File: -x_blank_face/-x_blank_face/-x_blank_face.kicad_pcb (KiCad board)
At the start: 2 copper layers, 87 x 326.5 mm, 29 parts, among them J1 Conn_01x08_Pin, J2 Conn_01x02_Pin, J3 Conn_01x02_Pin

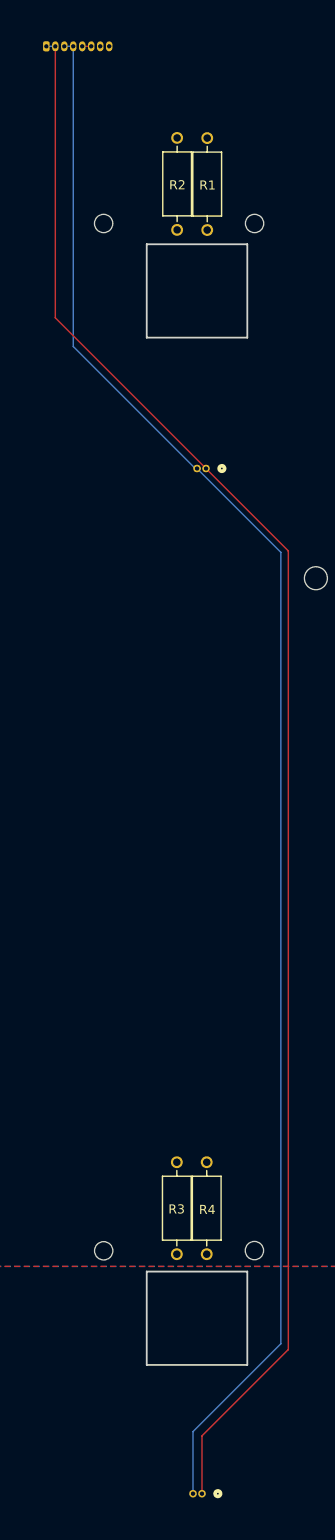
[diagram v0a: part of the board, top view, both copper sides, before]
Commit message: Rerouted some stuff
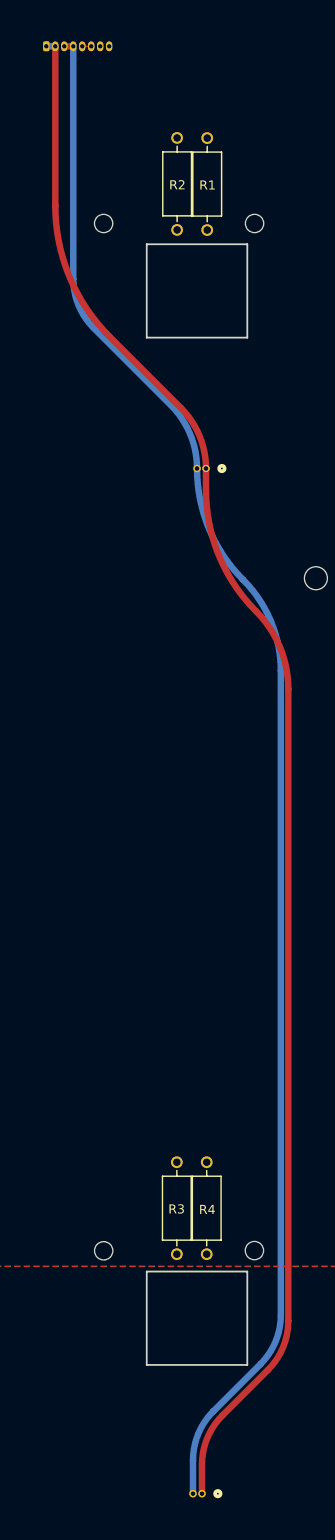
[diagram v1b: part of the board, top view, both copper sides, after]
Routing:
- net GND: track 221.4 -> 216.8 mm
- net /-X Serial Out: track 219.9 -> 215.8 mm
